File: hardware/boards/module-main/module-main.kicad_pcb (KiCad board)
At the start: 4 copper layers, 48.5 x 108.5 mm, 177 parts, among them J1 2x8 2.54mm shrouded box heade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, J2 2x10 2.54mm pin header, J3 Neutrik NE8FAV, J4 JST B2B-XH-A, Q1 PSMN2R0-30YLE, SW1 NKK M2011SD4G01, U1 LT3042EMSE, U10 OPA2197, U11 OPA2197, U12 OPA2197, U13 ADP7118AUJZ-5.0, U14 RPA20-2412SAW, U15 74AHCT14, U2 LT1641-1IS8, U3 DAC8568ICPW, U4 74AHCT125, U5 OPA2197, U6 INA828IDR, U7 OPA2197, U8 OPA2197IDR, U9 OPA2197

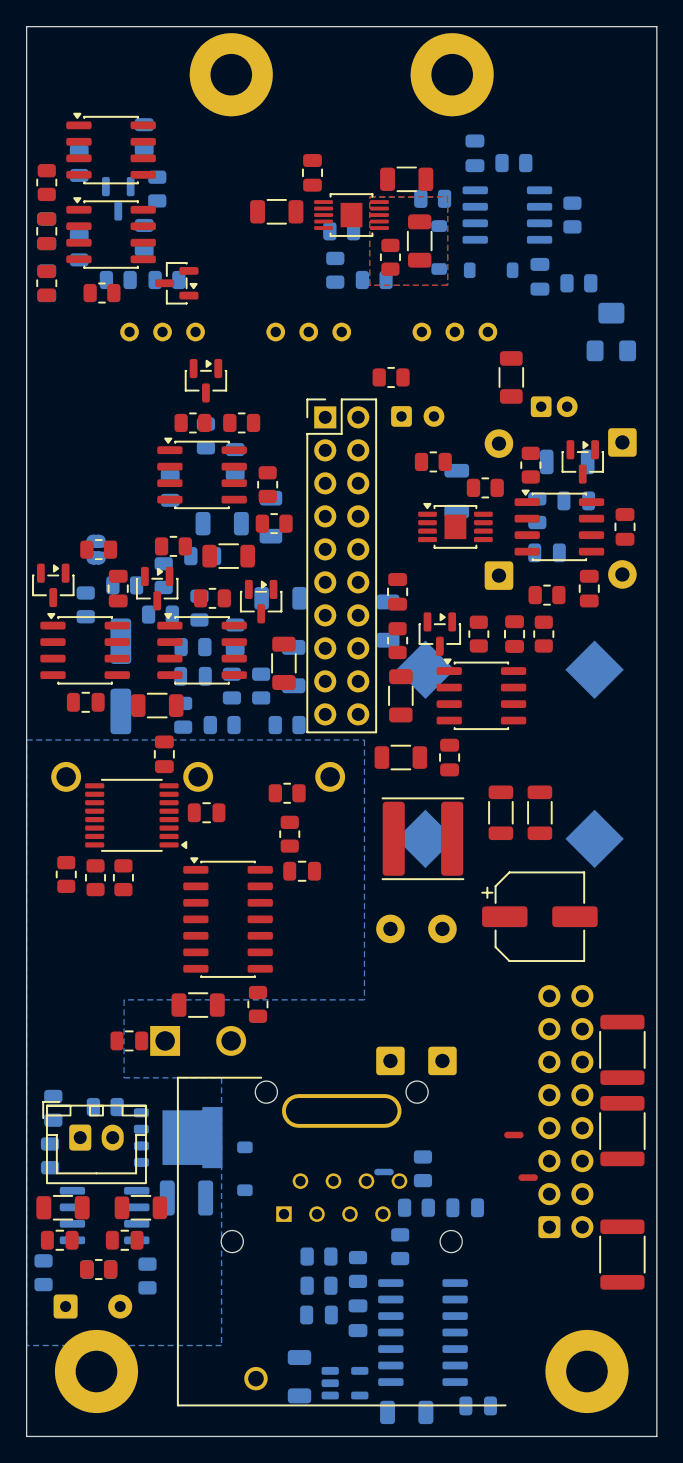
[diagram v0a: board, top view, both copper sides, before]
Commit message: module-main: routing in progress (resumable run's saved state)
Co-Authored-By: Claude Opus 5.5 <noreply@anthropic.com>
Claude-Session: https://claude.ai/code/session_01LmB4muFXnoLprWX4JzuJ5A
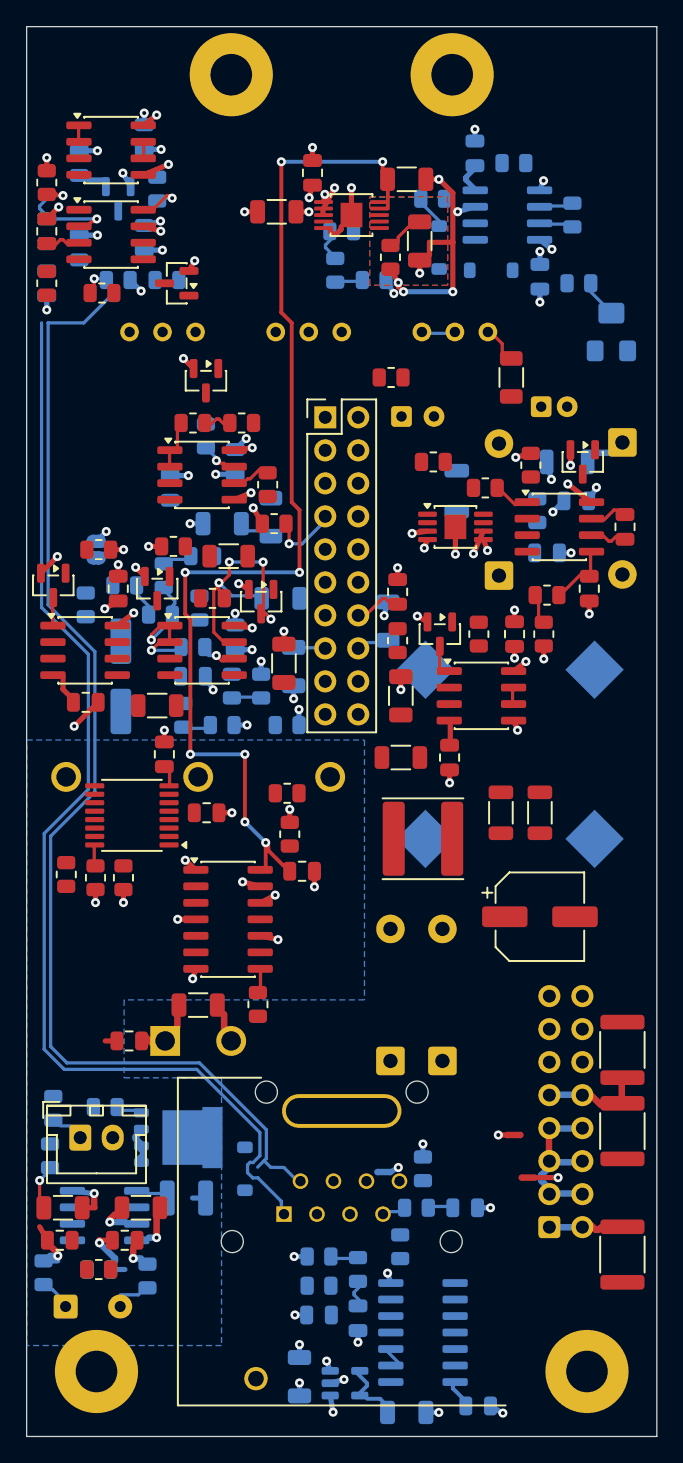
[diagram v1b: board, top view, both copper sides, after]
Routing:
- net /AGND_SENSE: track 0.00 -> 89.5 mm
- net AGND_MOD: track 0.00 -> 86.1 mm, vias 0 -> 59
- net /BREATH_SENSE: track 0.00 -> 85.8 mm
- net /DAC_AVDD: track 0.00 -> 80.7 mm, vias 0 -> 8
- net MODULE_ANALOG_POS12: track 0.00 -> 38.7 mm, vias 0 -> 32
- net DIG_GND: track 0.00 -> 21.8 mm, vias 0 -> 21
- net /mod-channels/OUT_1: track 0.00 -> 18.8 mm, vias 0 -> 4
- net PWR_GND: track 0.00 -> 13.4 mm, vias 0 -> 3
- net /mod-channels/VREF_MOD: track 0.00 -> 8.21 mm, vias 0 -> 2
- net /breath-receive-stage/IN_NEG: track 0.00 -> 7.55 mm, vias 0 -> 2
- net MODULE_ANALOG_NEG12: track 0.00 -> 6.26 mm
- net /power-entry/BUS_GND: track 0.00 -> 5.73 mm
- net LOGIC_5V: track 0.00 -> 5.08 mm
- net /PITCH_JACK: track 0.00 -> 4.11 mm
- net /GAIN_FLOOR: track 0.00 -> 3.98 mm, vias 0 -> 1
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
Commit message: module-main: routing in progress (94 connections left); pcb_route.escape for fine-pitch pads
Co-Authored-By: Claude Opus 5.5 <noreply@anthropic.com>
Claude-Session: https://claude.ai/code/session_01LmB4muFXnoLprWX4JzuJ5A
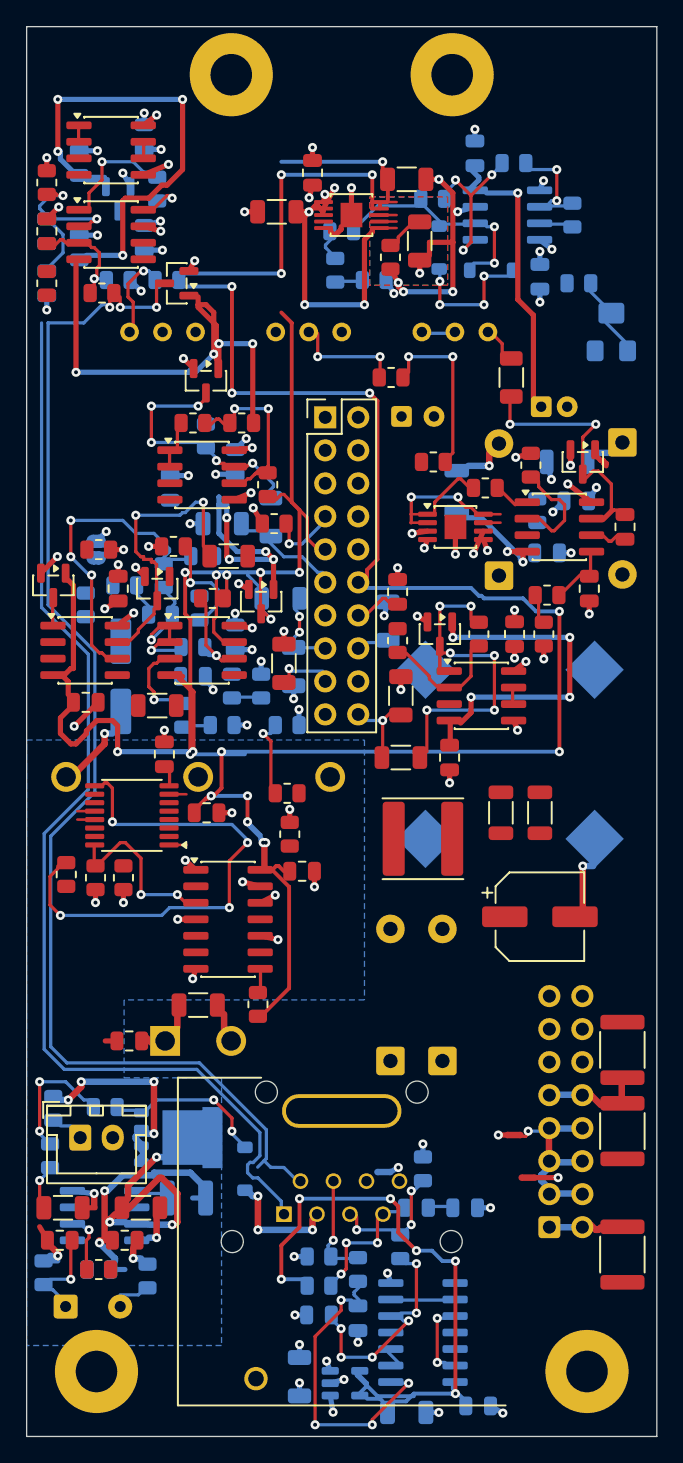
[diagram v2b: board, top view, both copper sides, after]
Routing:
- net MODULE_ANALOG_NEG12: track 6.26 -> 181.0 mm, vias 0 -> 21
- net /DAC_AVDD: track 80.7 -> 205.3 mm, vias 8 -> 18
- net LOGIC_5V: track 5.08 -> 49.5 mm, vias 0 -> 6
- net /dac8568/CLR: track 0.00 -> 38.0 mm, vias 0 -> 4
- net /mod-channels/OUT_4: track 1.00 -> 23.5 mm, vias 0 -> 6
- net /mod-channels/MINUS_3: track 1.00 -> 22.6 mm, vias 0 -> 3
- net /UMBILICAL_POS12: track 2.38 -> 23.7 mm, vias 0 -> 7
- net MODULE_ANALOG_POS12: track 38.7 -> 59.3 mm, vias 32 -> 34
- net /digital-and-supervision/SCLK_RC: track 1.33 -> 21.9 mm, vias 0 -> 4
- net /mod-channels/OUT_3: track 0.00 -> 19.7 mm, vias 0 -> 2
- net /pitch-stage/AMP_OUT: track 1.33 -> 18.7 mm, vias 0 -> 2
- net /digital-and-supervision/MOSI_RC: track 0.00 -> 15.6 mm, vias 0 -> 6
- net /umbilical-load-switch/SENSE_NODE: track 1.97 -> 16.5 mm, vias 1 -> 3
- net /breath-output-stage/BREATH_OUT: track 1.45 -> 15.8 mm, vias 1 -> 5
- net /pitch-stage/VREF_SUM: track 0.00 -> 12.3 mm, vias 0 -> 2
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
